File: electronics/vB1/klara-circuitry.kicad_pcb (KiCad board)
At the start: 2 copper layers, 70 x 39 mm, 15 parts, among them J1 Pin header, U1 MCP1700-3302E, U3 ATtiny85

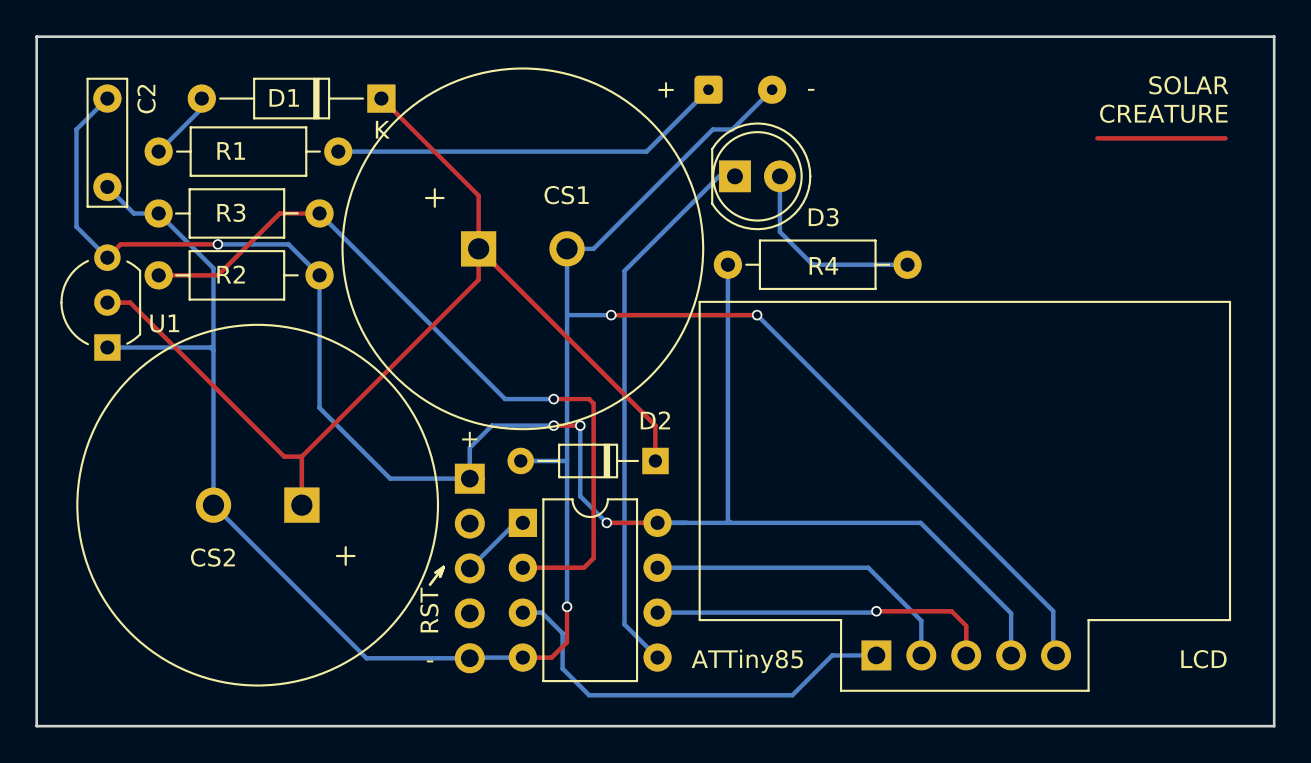
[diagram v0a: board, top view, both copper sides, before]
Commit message: PCB update
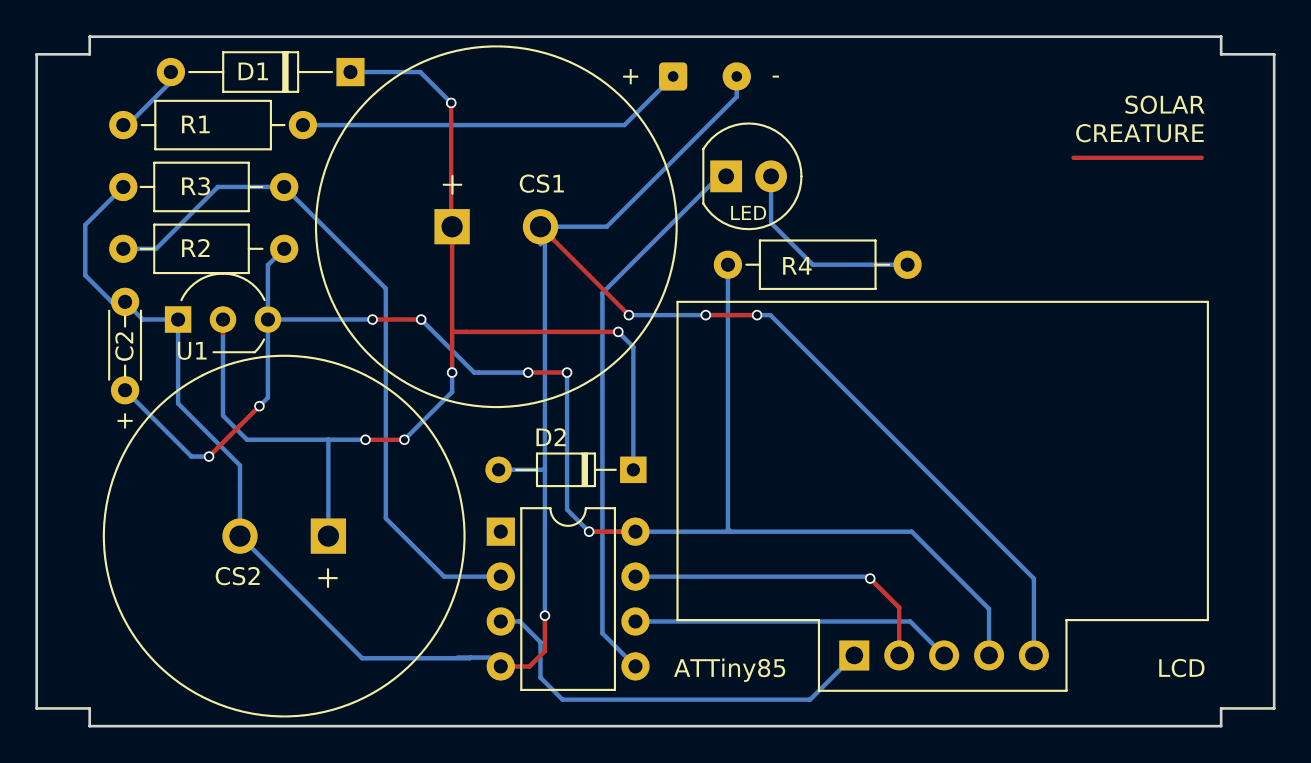
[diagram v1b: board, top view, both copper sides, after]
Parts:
- removed J1: Pin header, Connector_PinHeader_2.54mm:PinHeader_1x05_P2.54mm_Vertical
- moved C2 16.5 mm to (65.0, 93.0), turned to 90 degrees
- moved U1 4.30 mm to (68.0, 89.0), turned to 0 degrees
- moved R1 2.50 mm to (75.1, 78.0)
- moved R2 2.50 mm to (75.0, 85.0)
- moved R3 2.50 mm to (75.0, 81.5)
- moved CS2 2.30 mm to (76.5, 101.2)
- moved D1 2.30 mm to (77.8, 75.0)
- moved SC1 2.14 mm to (96.0, 75.2)
- moved CS1 1.95 mm to (83.5, 83.8)
- moved D2 1.35 mm to (93.8, 97.5)
- moved U3 1.35 mm to (86.2, 101.0)
- moved LCD 1.25 mm to (96.2, 110.0)
- moved LED 0.50 mm to (99.0, 80.9)
- renumbered D3 to LED
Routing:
- net Net-(C2-Pad1): track 100.2 -> 89.8 mm, vias 4 -> 7
- net Net-(CS1-Pad1): track 60.2 -> 66.7 mm, vias 0 -> 5
- net Net-(R2-Pad2): track 43.5 -> 39.5 mm, vias 1 -> 0
- net Net-(J1-Pad3): track 4.07 -> 0.42 mm
- net Net-(C2-Pad2): track 128.5 -> 131.8 mm, vias 3 -> 4
- net Net-(LCD1-Pad3): track 19.5 -> 18.3 mm, vias 1 -> 0
- net Net-(D3-Pad1): track 31.1 -> 32.1 mm
- net Net-(LCD1-Pad2): track 18.1 -> 18.5 mm, vias 0 -> 1
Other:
- outline, holes or cut-outs redrawn
- board text removed: "RST"
